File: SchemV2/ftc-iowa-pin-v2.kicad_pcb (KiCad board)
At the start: 2 copper layers, 37.9 x 24.3 mm, 62 parts, among them Q101 BSS84, Q102 BSS84, SW101 POWER, U101 TPS61220, U102 PIC16LF1704

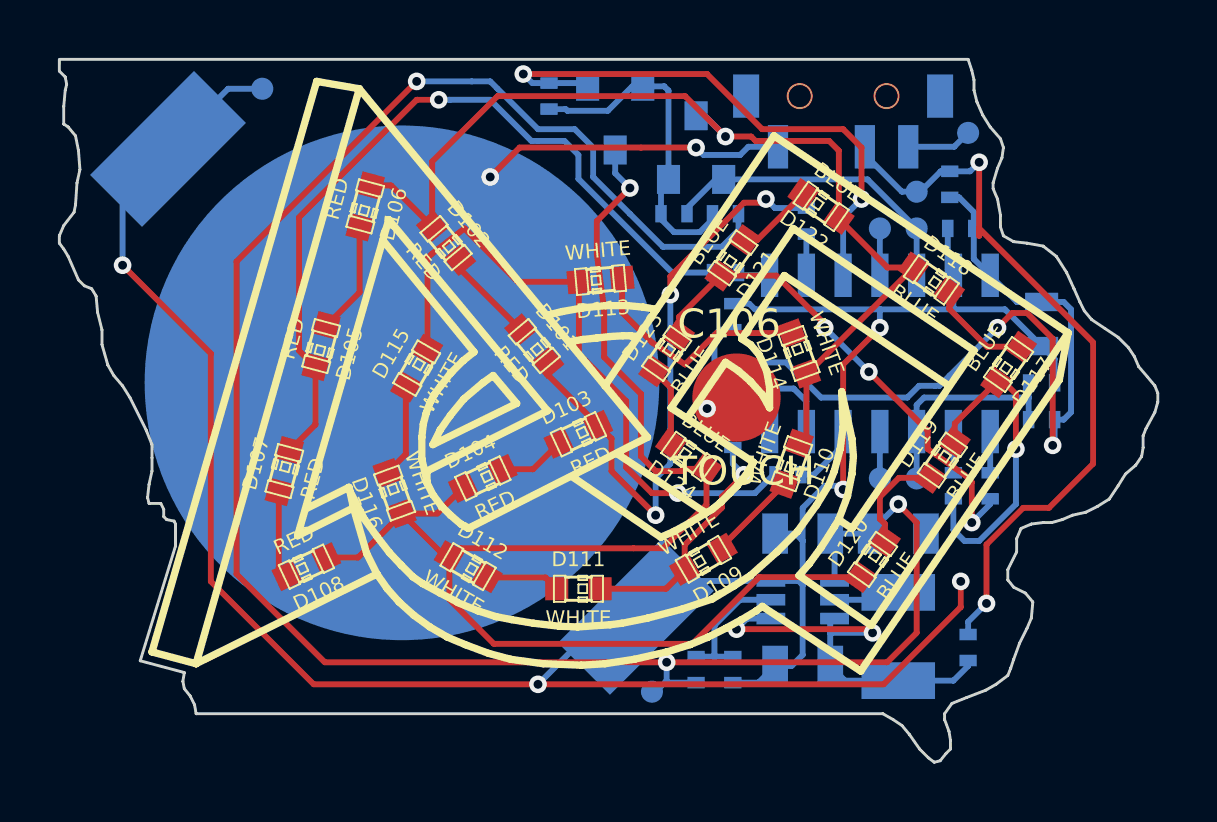
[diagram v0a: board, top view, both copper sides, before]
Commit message: cleaned up silk
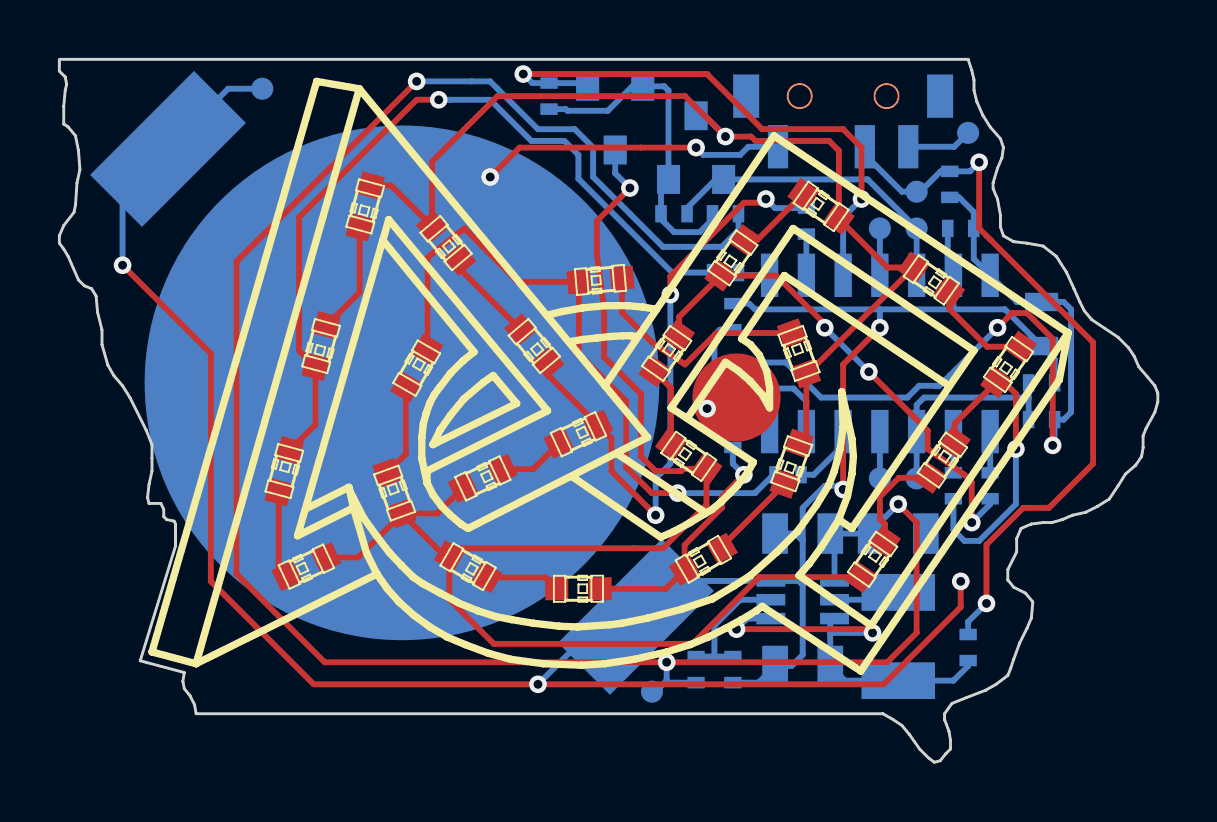
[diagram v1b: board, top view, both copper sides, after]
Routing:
- net /VSYS: track 25.9 -> 25.4 mm
